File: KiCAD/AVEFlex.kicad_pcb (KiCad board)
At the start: 2 copper layers, 19.6 x 29.7 mm, 35 parts, among them IC1 AVE-RVL

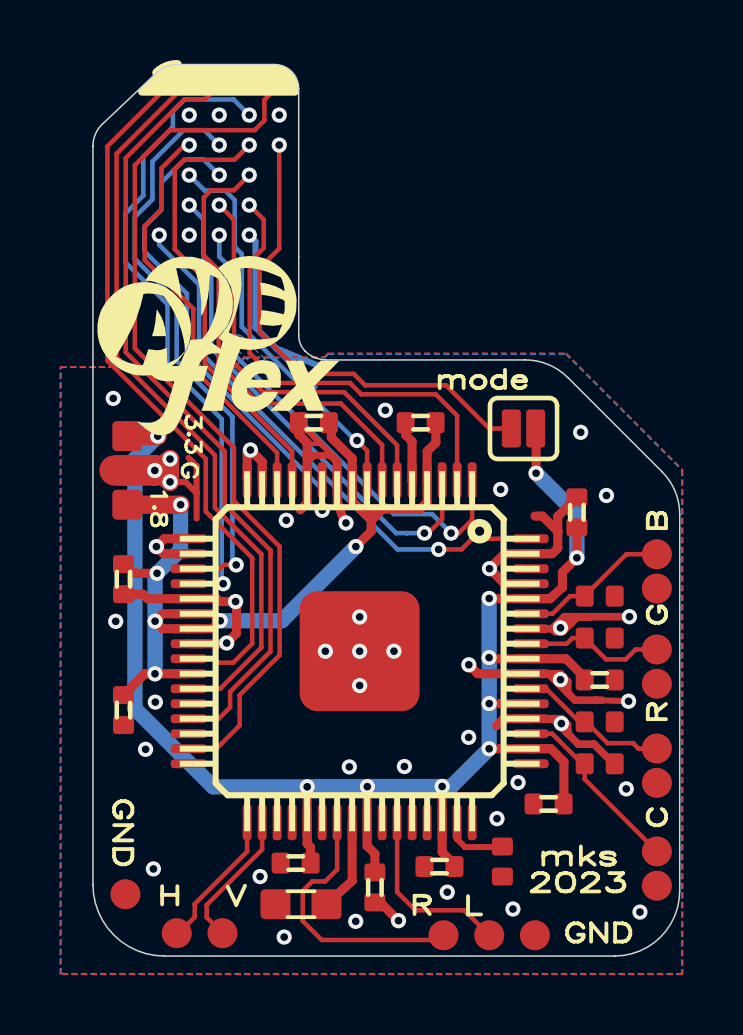
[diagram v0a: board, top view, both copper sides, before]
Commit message: Update KiCAD version
- updated KiCAD version
- updated Gerbers
- added new iBOM file
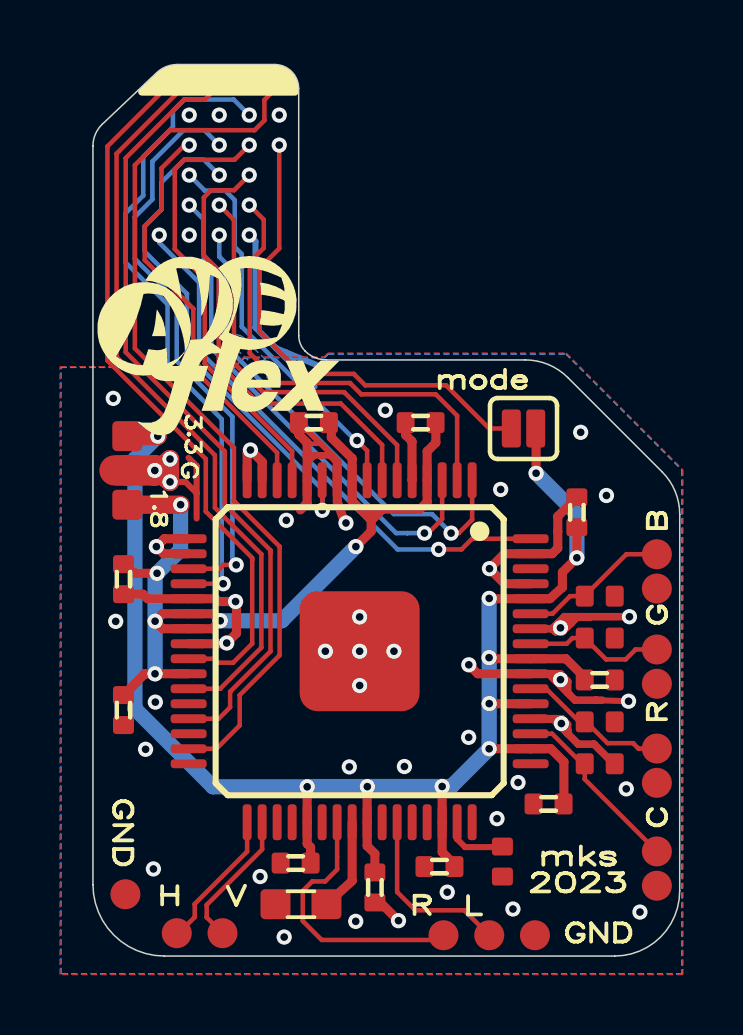
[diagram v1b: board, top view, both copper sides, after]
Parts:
- IC1: value AVE-RVL -> AVE
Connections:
- net B/PR renamed B/PR
- net G/PB renamed G/PB
- net IREF renamed Net-(IC1-IREF)
- net R/Y renamed R/Y
- IC1 pad 62: (no net) -> unconnected-(IC1-IPID-Pad62)
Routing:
- net GND: track 73.9 -> 71.3 mm
- net N$8: vias 1 -> 0
- net N$22: vias 1 -> 0
- net N$12: vias 1 -> 0
- net N$11: vias 1 -> 0
- net (no net): vias 0 -> 4
